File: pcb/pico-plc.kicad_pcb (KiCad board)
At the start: 2 copper layers, 154.5 x 95.5 mm, 172 parts, among them J1 Conn_02x06_Odd_Even, J12 Screw_Terminal_01x02, J13 Screw_Terminal_01x02, J15 Conn_01x03, J16 Conn_01x03, J18 Screw_Terminal_01x03, J19 Screw_Terminal_01x03, J2 Conn_01x06, J20 Screw_Terminal_01x03, J21 Screw_Terminal_01x03, J22 Screw_Terminal_01x03, J23 Screw_Terminal_01x03, J24 Screw_Terminal_01x03, J25 Screw_Terminal_01x03, J26 Screw_Terminal_01x02, J27 Screw_Terminal_01x02, J28 Screw_Terminal_01x02, J29 Screw_Terminal_01x02, J3 Conn_02x06_Odd_Even, J30 Screw_Terminal_01x02, J31 Screw_Terminal_01x02, J32 Screw_Terminal_01x02, J33 Screw_Terminal_01x02, J5 Conn_01x06, J6 Conn_01x06, J7 Screw_Terminal_01x02, J8 Conn_01x02, K1 Relay_SPDT, K2 Relay_SPDT, K3 Relay_SPDT, K4 Relay_SPDT, K5 Relay_SPDT, K6 Relay_SPDT, K7 Relay_SPDT, K8 Relay_SPDT, Q1 BSS138, Q10 NDS355AN, Q11 NDS355AN, Q12 NDS355AN, Q13 NDS355AN, Q14 NDS355AN, Q15 NDS355AN, Q2 BSS138, Q3 BSS138, Q4 BSS138, Q5 BSS138, Q6 BSS138, Q7 BSS138, Q8 NDS355AN, Q9 NDS355AN, U1 DS18B20, U2 VO615A, U3 VO615A, U4 VO615A, U5 VO615A, U6 VO615A, U7 VO615A, U8 VO615A, U9 VO615A

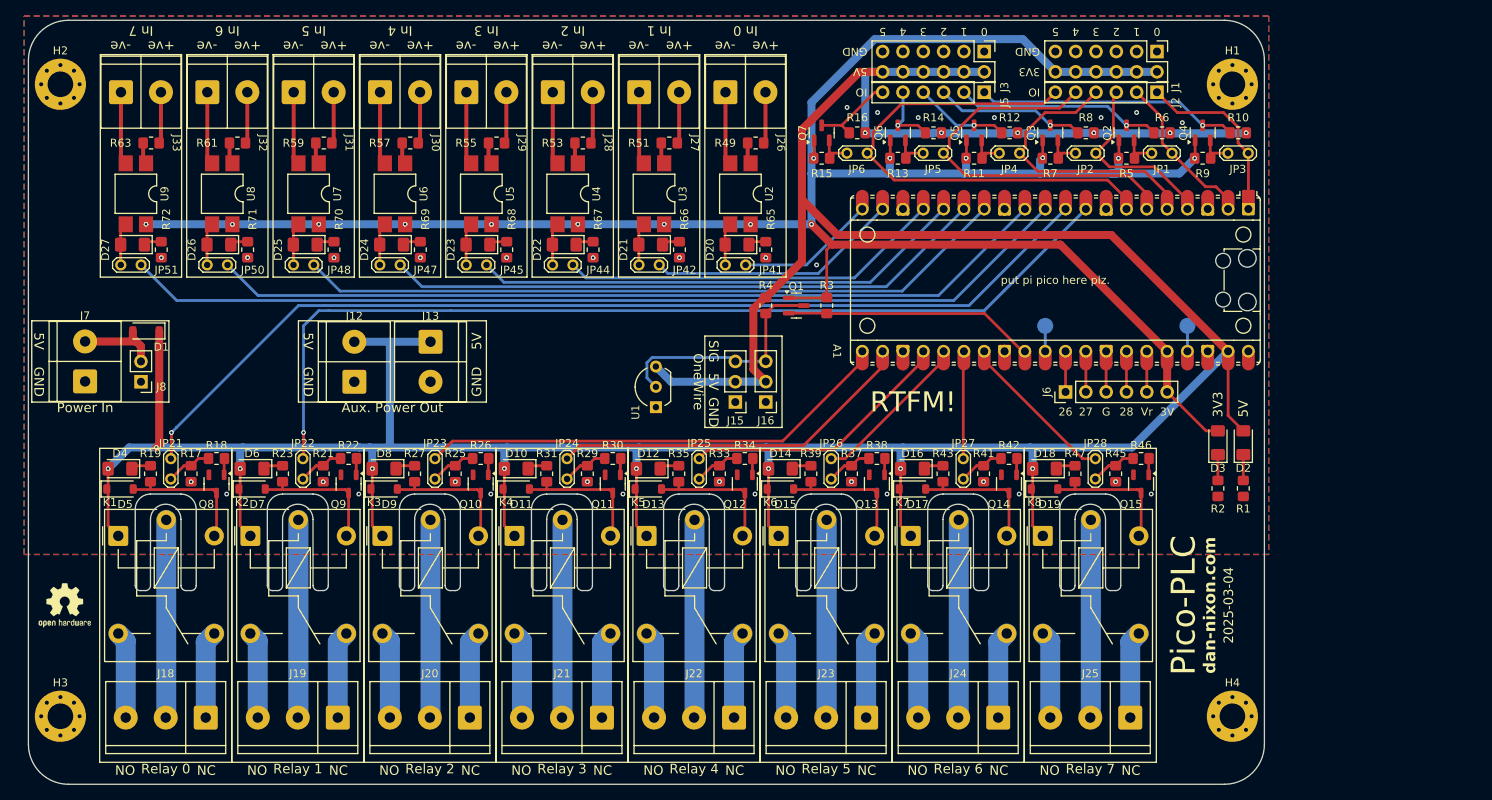
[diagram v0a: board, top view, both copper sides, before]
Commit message: New board revision
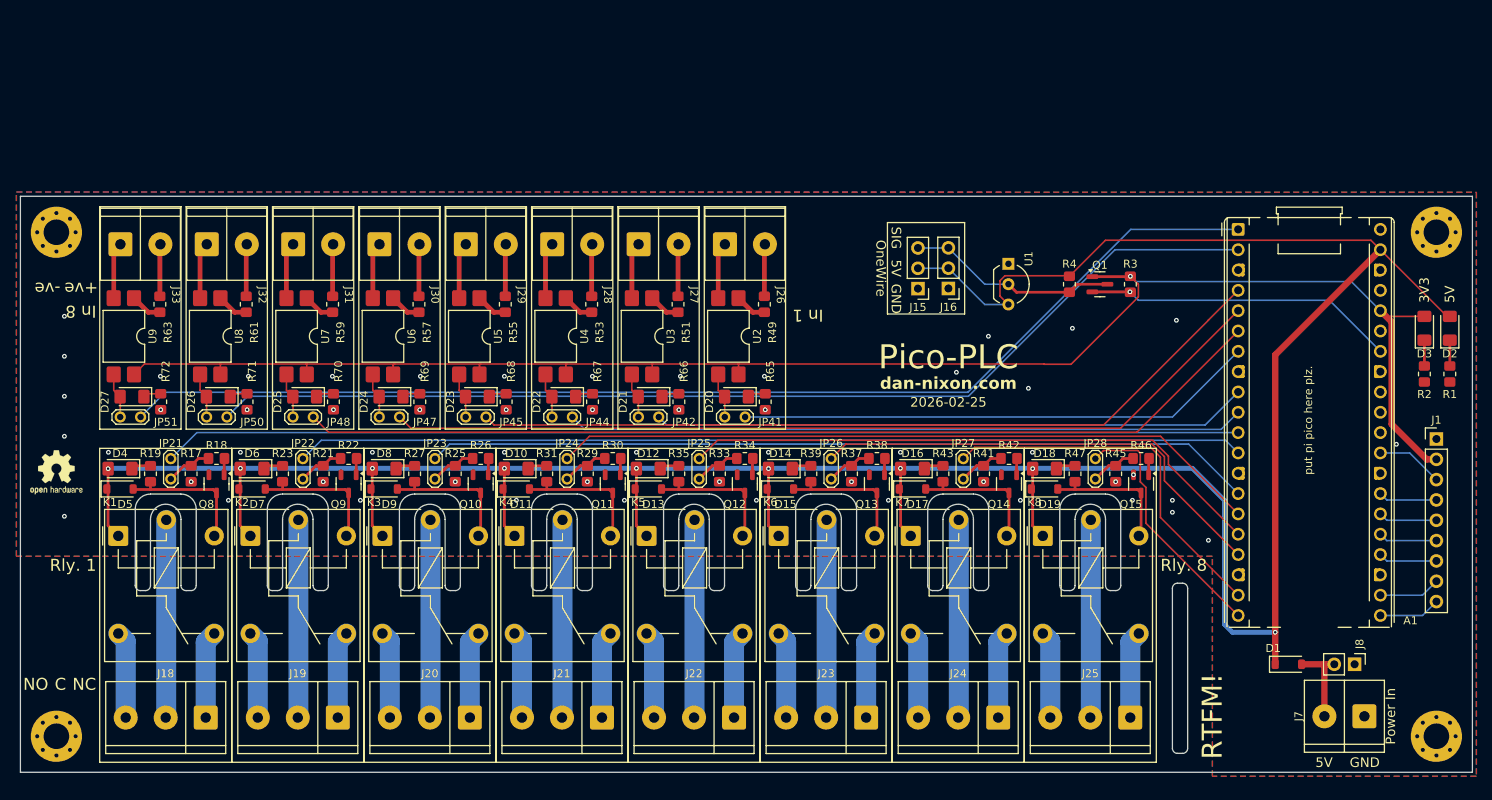
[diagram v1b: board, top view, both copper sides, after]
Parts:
- removed J12, J13: Screw_Terminal_01x02, Conn_ScrewTerminals:CTB7000-2
- removed J2, J5, J6: Conn_01x06, Connector_PinHeader_2.54mm:PinHeader_1x06_P2.54mm_Vertical
- removed J3: Conn_02x06_Odd_Even, Connector_PinHeader_2.54mm:PinHeader_2x06_P2.54mm_Vertical
- removed JP1, JP2, JP3, JP4, JP5, JP6: Jumper_2_Open, TestPoint:TestPoint_2Pads_Pitch2.54mm_Drill0.8mm
- removed Q2, Q3, Q4, Q5, Q6, Q7: BSS138, Package_TO_SOT_SMD:SOT-23
- removed R10, R11, R12, R13, R14, R15, R16, R5, R6, R7, R8, R9: 10k, Resistor_SMD:R_0805_2012Metric_Pad1.20x1.40mm_HandSolder
- removed TP1: Run, TestPoint:TestPoint_Pad_D2.0mm
- removed TP2: 3.3V En, TestPoint:TestPoint_Pad_D2.0mm
- A1: footprint RaspberryPi_Pico:RaspberryPi_Pico_Common -> Module:RaspberryPi_Pico_Common_THT
- J1: value Conn_02x06_Odd_Even -> Conn_01x09; footprint Connector_PinHeader_2.54mm:PinHeader_2x06_P2.54mm_Vertical -> Connector_PinHeader_2.54mm:PinHeader_1x09_P2.54mm_Vertical
- U2, U3, U4, U5, U6, U7, U8, U9: footprint Package_DIP:SMDIP-4_W7.62mm -> Package_DIP:SMDIP-4_W9.53mm
- moved J7 163.5 mm to (202.5, 125.0), turned to 0 degrees
- moved J8 155.8 mm to (203.8, 118.5), turned to -90 degrees
- moved D1 148.7 mm to (195.5, 118.5), turned to 0 degrees
- moved J1 59.7 mm to (214.0, 90.3), turned to 0 degrees
- moved U1 47.6 mm to (160.5, 68.4), turned to -90 degrees
- moved R3 38.0 mm to (175.7, 71.0)
- moved Q1 38.0 mm to (171.9, 71.0)
- moved R4 38.0 mm to (168.1, 71.0)
- moved H1 31.5 mm to (214.0, 64.5)
- moved D2 29.5 mm to (215.7, 76.5)
- moved D3 29.5 mm to (212.5, 76.5)
- moved R1 29.5 mm to (215.7, 82.2)
- moved R2 29.5 mm to (212.5, 82.2)
- moved J15 26.9 mm to (149.2, 71.5)
- moved J16 26.9 mm to (153.0, 71.5)
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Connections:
- A1 pad 30: /RUN -> unconnected-(A1-RUN-Pad30)
- A1 pad 31: /IO26 -> unconnected-(A1-GPIO26_ADC0-Pad31)
- A1 pad 32: /IO27 -> unconnected-(A1-GPIO27_ADC1-Pad32)
- A1 pad 33: GNDA -> unconnected-(A1-AGND-Pad33)
- A1 pad 35: /ADC_VREF -> unconnected-(A1-ADC_VREF-Pad35)
- A1 pad 37: /3V3_EN -> unconnected-(A1-3V3_EN-Pad37)
- J1 pad 3: GND -> /IO22
- J1 pad 4: +3V3 -> /IO21
- J1 pad 5: GND -> /IO20
- J1 pad 6: +3V3 -> /IO19
- J1 pad 7: GND -> /IO18
- J1 pad 8: +3V3 -> /IO17
- J1 pad 9: GND -> /IO16
- JP21 pad 1: /IO7 -> /IO8
- JP22 pad 1: /IO6 -> /IO9
- JP23 pad 1: /IO16 -> /IO10
- JP24 pad 1: /IO17 -> /IO11
- JP25 pad 1: /IO18 -> /IO12
- JP26 pad 1: /IO19 -> /IO13
- JP27 pad 1: /IO20 -> /IO14
- JP28 pad 1: /IO21 -> /IO15
- JP41 pad 2: /IO15 -> /IO5
- JP42 pad 2: /IO14 -> /IO6
- JP44 pad 2: /IO13 -> /IO7
- JP45 pad 2: /IO12 -> /IO2
- JP47 pad 2: /IO11 -> /IO3
- JP48 pad 2: /IO10 -> /IO4
- JP50 pad 2: /IO9 -> /IO1
- JP51 pad 2: /IO8 -> /IO0
- Q1 pad 2: /IO22 -> /IO28
- R3 pad 2: /IO22 -> /IO28
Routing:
- net /IO0: track 22.7 -> 146.9 mm
- net /IO1: track 20.1 -> 135.1 mm
- net +5V: track 475.8 -> 371.1 mm, vias 15 -> 9
- net +3V3: track 293.7 -> 207.6 mm, vias 15 -> 1
- net /IO2: track 23.7 -> 101.4 mm
- net /IO3: track 36.3 -> 111.5 mm
- net /IO4: track 49.8 -> 121.6 mm
- net /IO16: track 59.7 -> 7.72 mm
- net /IO6: track 120.5 -> 74.6 mm, vias 1 -> 0
- net /IO7: track 126.6 -> 84.8 mm, vias 1 -> 0
- net /IO17: track 46.1 -> 7.72 mm
- net /IO28: track 5.08 -> 39.1 mm, vias 0 -> 1
- net /General IO/IO0_SHIFTED: track 32.9 -> 0.00 mm, vias 1 -> 0
- net /IO18: track 34.2 -> 7.33 mm
- net /General IO/IO1_SHIFTED: track 25.9 -> 0.00 mm, vias 1 -> 0
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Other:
- board size 154.5 x 95.5 mm -> 181.5 x 72 mm
- board text added: "2026-02-25"
- board text added: "C"
- board text added: "In 8"
- board text added: "M3 mounting holes Hole centres: 172.5 x 63 Board size: 181.5 x 72"
- board text added: "Rly. 1"
- board text added: "Rly. 8"
- board text removed: "0"
- board text removed: "1"
- board text removed: "2"
- board text removed: "2025-03-04"
- board text removed: "26"
- board text removed: "27"
- board text removed: "28"
- board text removed: "3"
- board text removed: "3V"
- board text removed: "3V3_EN"
- board text removed: "4"
- board text removed: "5"
- board text removed: "Aux. Power Out"
- board text removed: "G"
- board text removed: "IO"
- board text removed: "In 0"
- board text removed: "In 2"
- board text removed: "In 3"
- board text removed: "In 4"
- board text removed: "In 5"
- board text removed: "In 6"
- board text removed: "In 7"
- board text removed: "JLCJLCJLCJLC"
- board text removed: "M3 mounting holes"
- board text removed: "RUN"
- board text removed: "Relay 0"
- board text removed: "Relay 1"
- board text removed: "Relay 2"
- board text removed: "Relay 3"
- board text removed: "Relay 4"
- board text removed: "Relay 5"
- board text removed: "Relay 6"
- board text removed: "Relay 7"
- board text removed: "Vr"
